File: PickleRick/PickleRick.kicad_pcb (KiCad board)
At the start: 4 copper layers, 100 x 37 mm, 176 parts, among them J1 Conn_01x06_Male, J10 Conn_01x03_Male, J11 Conn_01x02_Male, J12 Conn_01x05_Male, J14 DeployLipo, J15 UCLipo, J16 Conn_Coaxial, J17 USB_C_Receptacle_USB2.0, J18 Conn_Coaxial, J2 Conn_01x02_Male, J3 Conn_01x02_Male, J4 Micro_SD_Card_Det, J5 CON7_1X7_DRH_HPI125_TYC, J6 Screw_Terminal_01x08, Q1 MMDT2222A, Q10 AO3401A, Q2 PMV20ENR, Q3 NCV8415STT1G, Q4 NCV8415STT1G, Q5 NCV8415STT1G, Q6 NCV8415STT1G, Q7 SI4143DY-T1-GE3, Q8 SI4143DY-T1-GE3, Q9 AO3401A, U1 SN65HVD230, U10 LTC4411ES5TRMPBF, U11 LTC4411ES5TRMPBF, U12 LT1963AxST-3.3, U13 LTC4412xS6, U14 LTC4412xS6, U15 LTC4412xS6, U16 LTC4412xS6, U17 MAX-M8Q, U18 CP2102-GMR-QFN28, U19 RFM95W-868S2, U2 ESP32-WROOM-32D, U3 MS5607-02BA, U4 LTV-247, U5 PCA9534RGVR, U6 PCA9685BS, U7 H3LIS100DLTR, U8 ICM-20608-G, U9 MMC5983MA

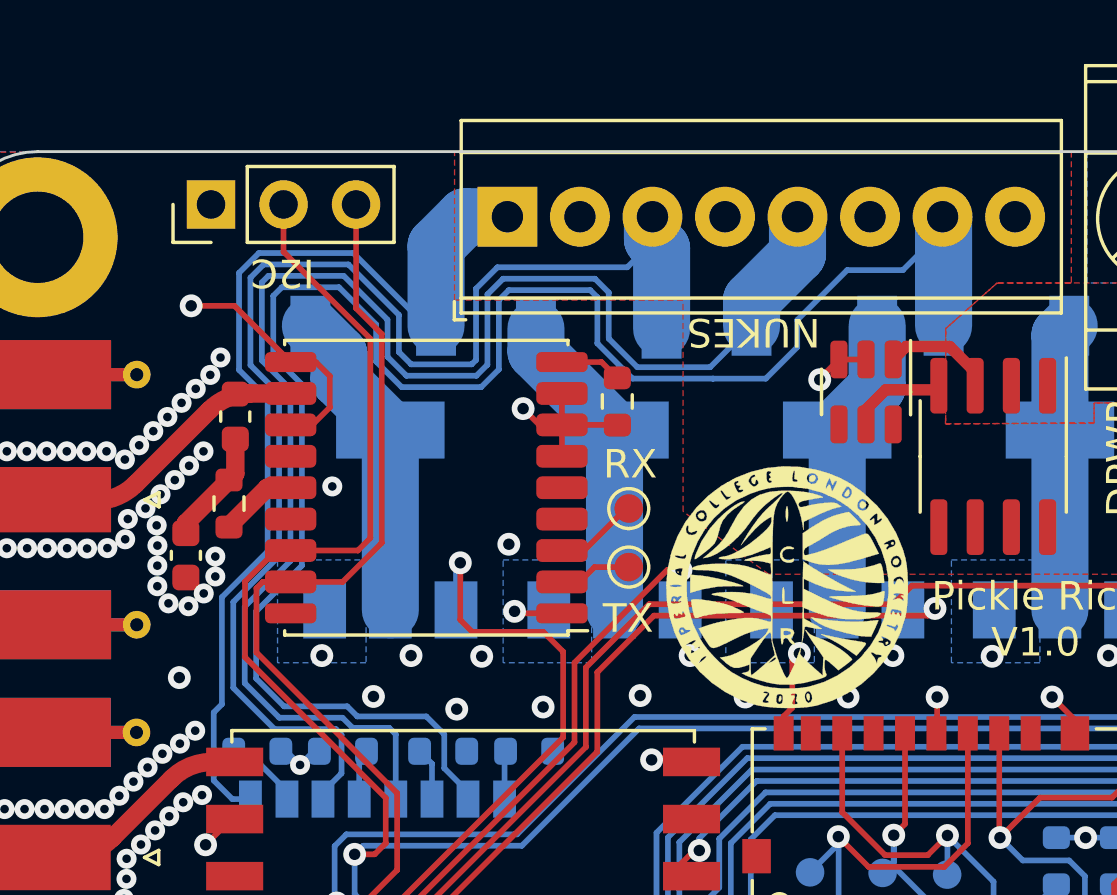
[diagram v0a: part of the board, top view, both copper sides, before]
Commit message: pcikle
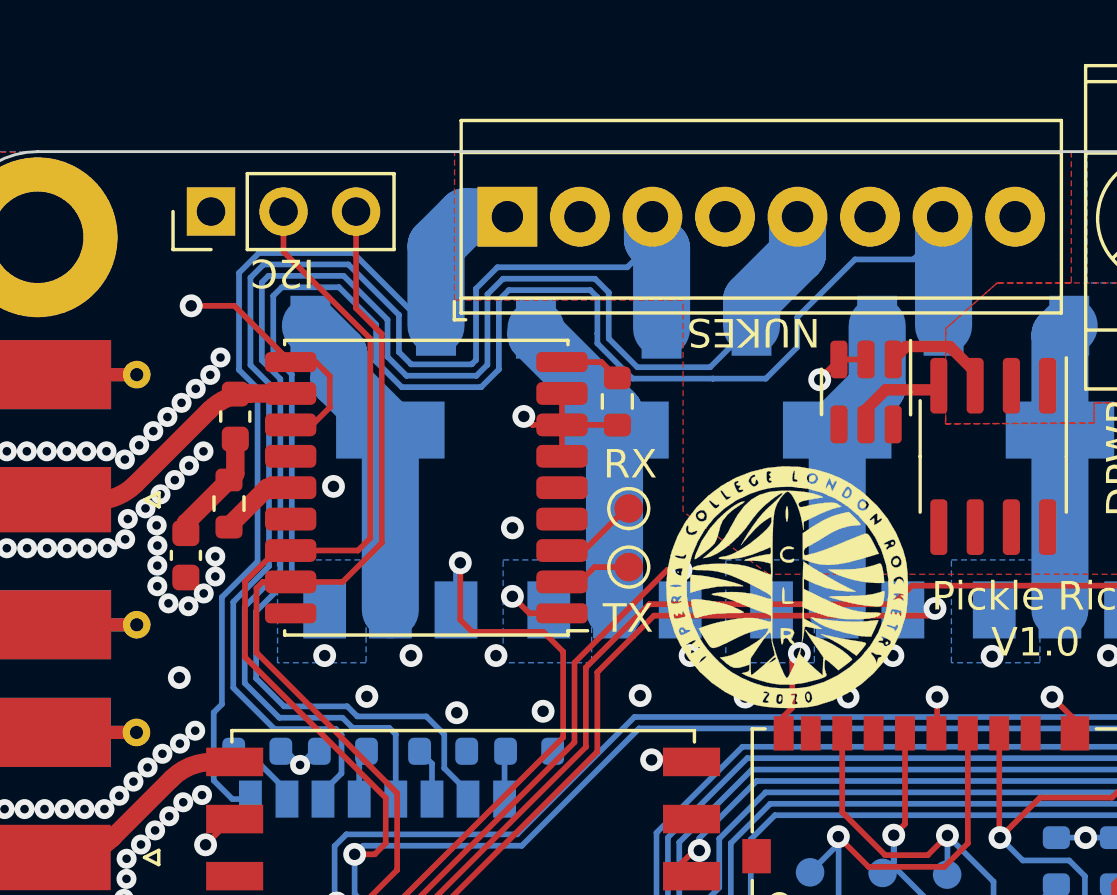
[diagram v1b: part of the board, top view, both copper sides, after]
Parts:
- moved J10 0.25 mm to (109.1, 62.1)
